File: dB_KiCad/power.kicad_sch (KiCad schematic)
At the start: 1 part

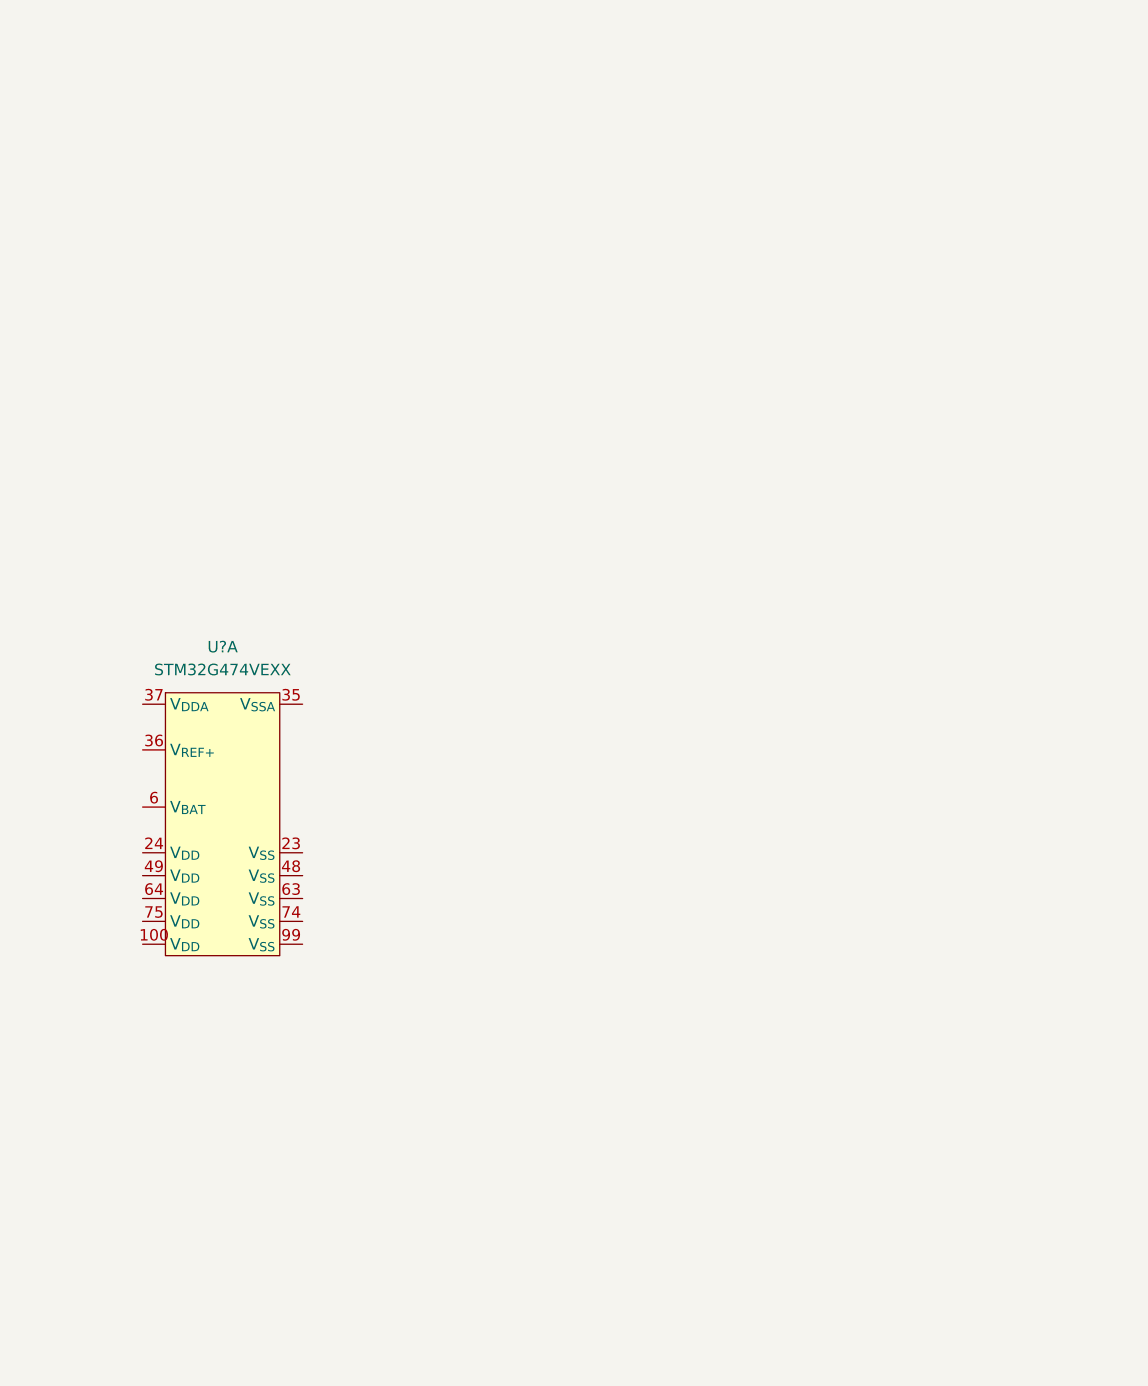
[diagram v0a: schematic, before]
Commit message: buck converter
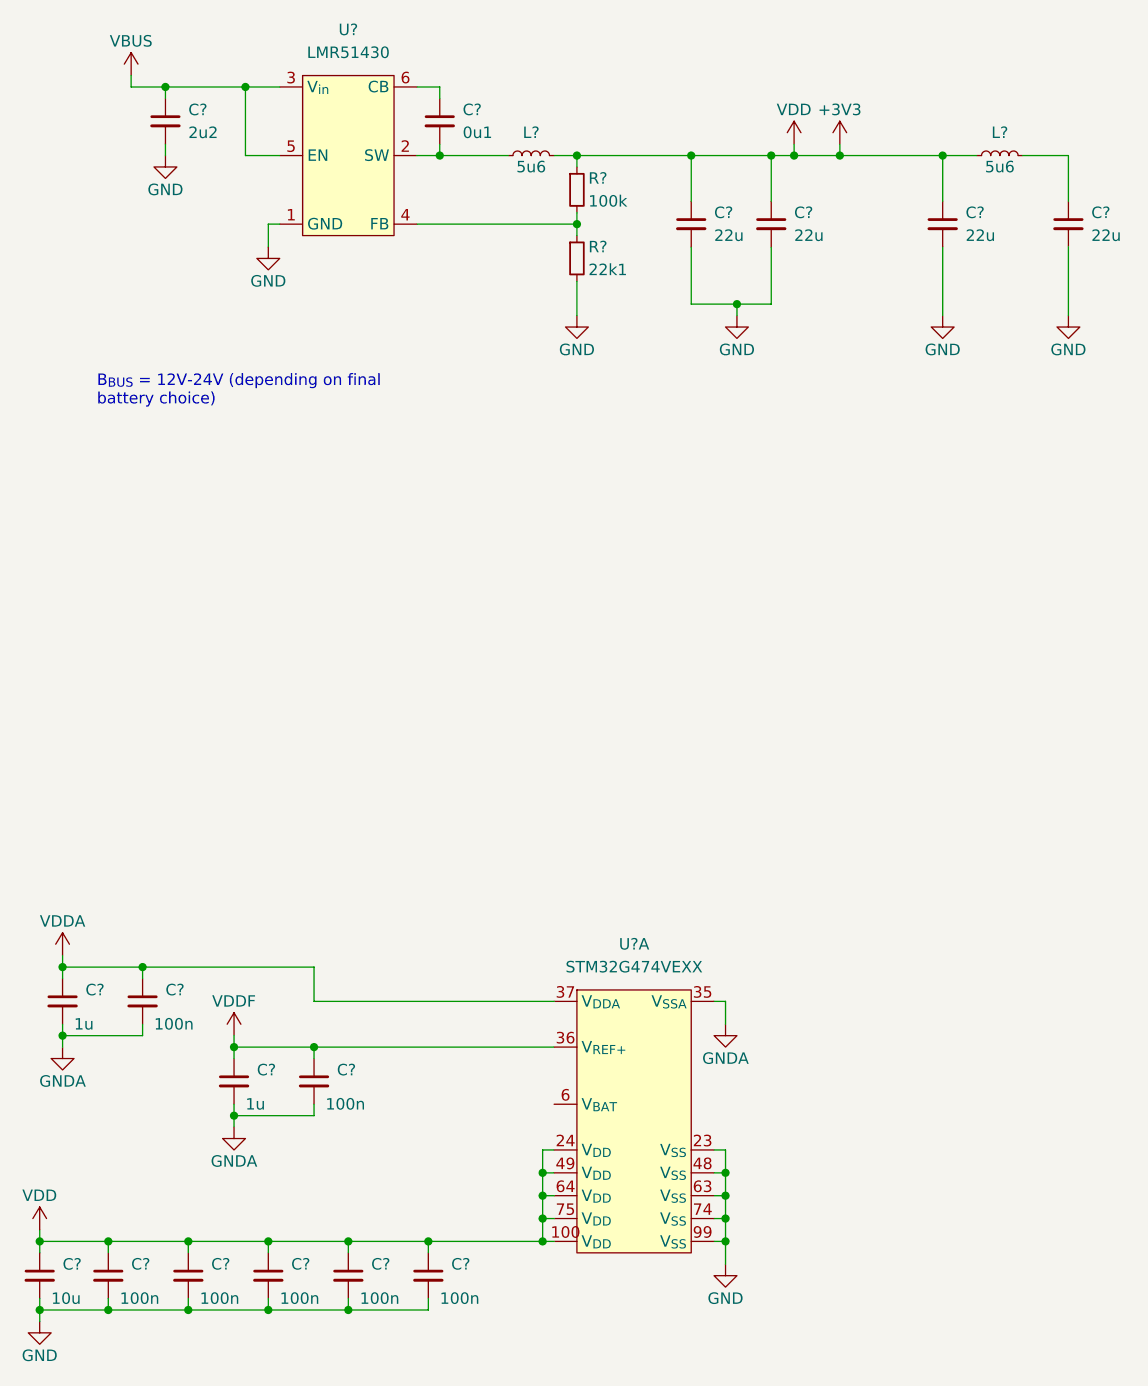
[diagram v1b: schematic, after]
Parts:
- added C? (x2): 1u, symbol Device:C_Small
- added C? (x7): 100n, symbol Device:C_Small
- added C?: 2u2, symbol Device:C_Small
- added C? (x4): 22u, symbol Device:C_Small
- added C?: 10u, symbol Device:C_Small
- added C?: 0u1, symbol Device:C_Small
- added L? (x2): 5u6, symbol Device:L_Small
- added R?: 100k, symbol Device:R_Small
- added R?: 22k1, symbol Device:R_Small
- added U?: LMR51430, Package_TO_SOT_SMD:SOT-23-6, symbol additional_lib:LMR51430
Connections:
- net +3V3: now reaches U?.100 (V_{DD})
- net +3V3: now also U?.24 (V_{DD}), U?.49 (V_{DD}), U?.64 (V_{DD}), U?.75 (V_{DD}), C?.1, C?.1, C?.1, C?.1, C?.1, C?.1, C?.1, C?.1, C?.1, L?.1, L?.2, R?.1
- net GND: now reaches U?.23 (V_{SS})
- net GND: now also U?.48 (V_{SS}), U?.63 (V_{SS}), U?.74 (V_{SS}), U?.99 (V_{SS}), C?.2, C?.2, C?.2, C?.2, C?.2, C?.2, C?.2, C?.2, C?.2, C?.2, C?.2, R?.2, U?.1 (GND)
- net GNDA: now reaches U?.35 (V_{SSA})
- net GNDA: now also C?.2, C?.2, C?.2, C?.2
- net VDDF: now reaches U?.36 (V_{REF+})
- net VDDF: now also C?.1, C?.1
- net VDDA: now reaches U?.37 (V_{DDA})
- net VDDA: now also C?.1, C?.1
- new net: R?.1, R?.2, U?.4 (FB)
- new net: C?.1, L?.2
- new net: C?.2, L?.1, U?.2 (SW)
- new net: C?.1, U?.6 (CB)
- new net VBUS: C?.1, U?.3 (V_{in}), U?.5 (EN)
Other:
- note added: "B_{BUS} = 12V-24V (depending on final battery choice)"
- moved on the sheet: U?A
